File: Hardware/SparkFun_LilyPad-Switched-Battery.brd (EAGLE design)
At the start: 29.8 x 29.7 mm, 13 parts

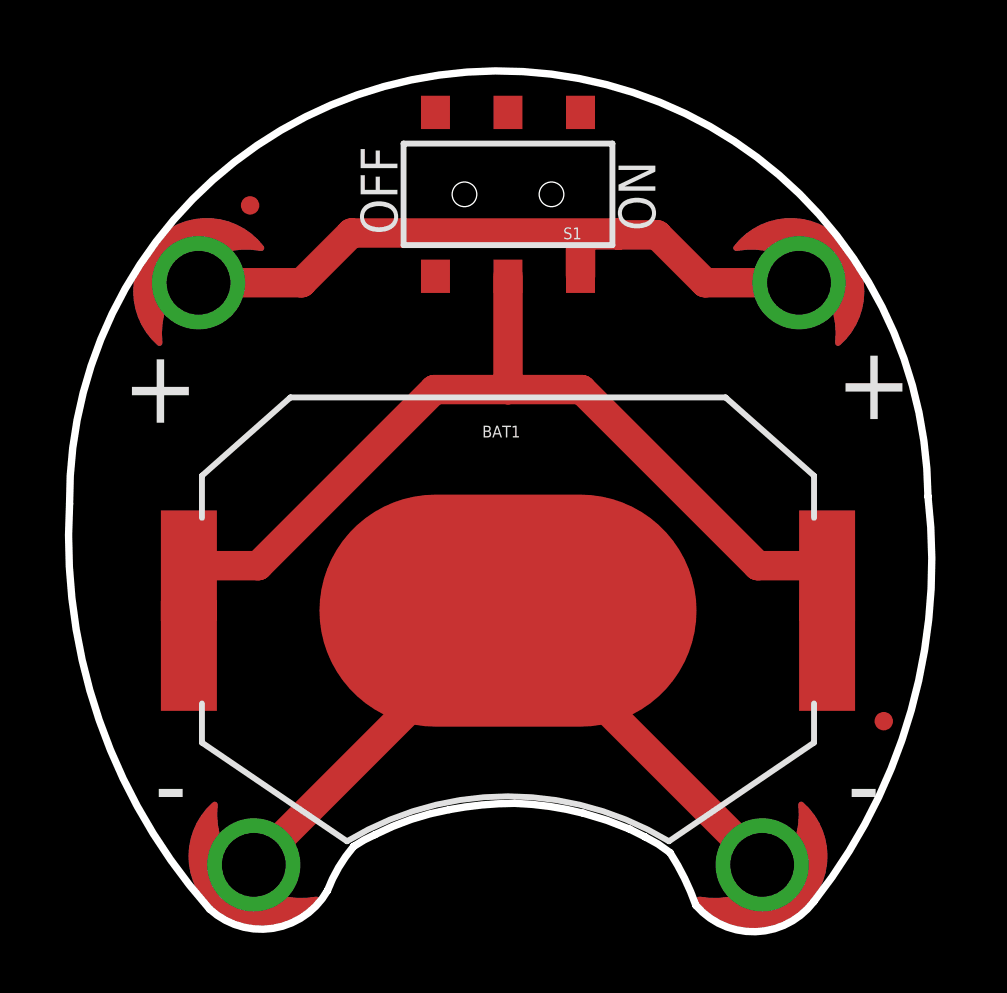
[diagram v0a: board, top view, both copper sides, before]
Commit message: updated board and schematic files
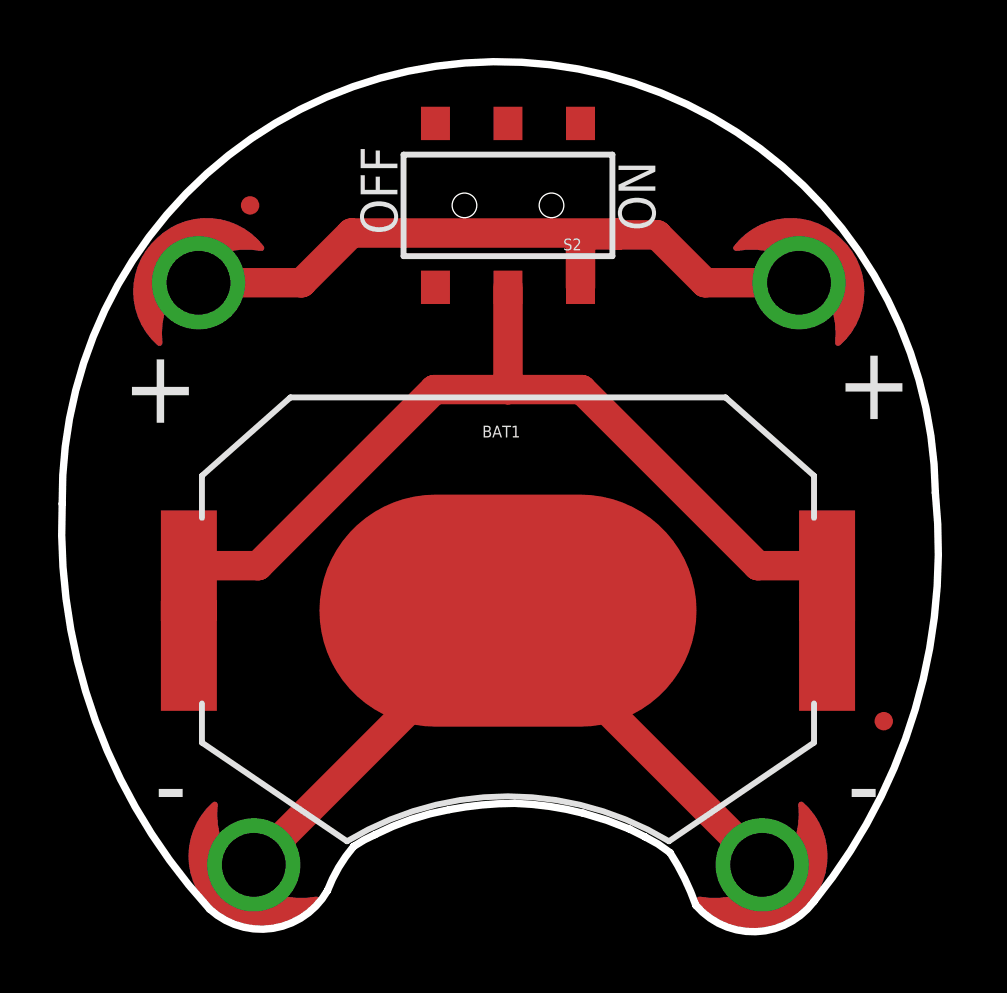
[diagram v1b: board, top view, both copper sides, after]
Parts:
- removed S1: Switch, SparkFun:AYZ0202
- added S2: (no value), SparkFun-Electromechanical:AYZ0202
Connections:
- net N$1: now also S2.1; no longer S1.1
- net N$3: now also S2.2; no longer S1.2
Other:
- board size 29.8 x 29.7 mm -> 30.2 x 30 mm
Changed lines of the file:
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@@
 <setting verticaltext="up"/>
 </settings>
-<grid distance="0.0125" unitdist="inch" unit="inch" style="lines" multiple="1" display="yes" altdistance="0.005" altunitdist="inch" altunit="inch"/>
+<grid distance="0.05" unitdist="inch" unit="inch" style="lines" multiple="1" display="yes" altdistance="0.005" altunitdist="inch" altunit="inch"/>
 <layers>
 <layer number="1" name="Top" color="4" fill="1" visible="yes" active="yes"/>
@@
 <text x="19.05" y="26.924" size="1.27" layer="21" font="vector" ratio="15" rot="R270">ON</text>
 <text x="10.16" y="27.432" size="1.27" layer="21" font="vector" ratio="15" rot="R270">OFF</text>
-<wire x1="0.127" y1="15.113" x2="4.953" y2="1.143" width="0.254" layer="20" curve="45"/>
+<wire x1="-0.127" y1="15.113" x2="4.953" y2="1.143" width="0.254" layer="20" curve="45"/>
 <wire x1="4.953" y1="1.143" x2="9.017" y2="1.778" width="0.254" layer="20" curve="103.204965"/>
 <wire x1="9.017" y1="1.778" x2="9.9187" y2="3.302" width="0.254" layer="20" curve="-19.629056"/>
@@
 <wire x1="17.8435" y1="4.445" x2="19.431" y2="3.8989" width="0.254" layer="20" curve="-8.804635"/>
 <wire x1="19.9644" y1="3.6322" x2="20.828" y2="3.0861" width="0.254" layer="20" curve="-13.702835"/>
-<wire x1="29.718" y1="15.367" x2="0.127" y2="15.113" width="0.254" layer="20" curve="180"/>
-<wire x1="29.718" y1="15.367" x2="25.781" y2="1.397" width="0.254" layer="20" curve="-45"/>
+<wire x1="29.972" y1="15.494" x2="-0.127" y2="15.113" width="0.254" layer="20" curve="180"/>
+<wire x1="29.972" y1="15.494" x2="25.781" y2="1.397" width="0.254" layer="20" curve="-45"/>
 <wire x1="25.781" y1="1.397" x2="21.717" y2="1.27" width="0.254" layer="20" curve="-102.203889"/>
 <wire x1="21.717" y1="1.27" x2="20.828" y2="3.0861" width="0.254" layer="20" curve="13.355078"/>
@@
 <element name="ST4" library="LilyPad-Wearables" package="PETAL-SMALL-2SIDE" value="SEWTAP6" x="25.273" y="22.733" rot="R137"/>
 <element name="U$5" library="LilyPad-Wearables" package="LOGO-LILYPAD" value="LOGO-LPLP" x="15.24" y="15.24" rot="MR0"/>
-<element name="S1" library="SparkFun" package="AYZ0202" value="Switch" x="15.24" y="25.781" rot="R180"/>
 <element name="BAT1" library="SparkFun-Electromechanical" package="BATTCON_20MM_4LEGS" value="20mm coincell" x="15.24" y="11.43">
 <attribute name="PROD_ID" value="BATT-10373" x="15.24" y="11.43" size="1.778" layer="27" display="off"/>
@@
 <element name="FRAME1" library="SparkFun-Aesthetics" package="CREATIVE_COMMONS" value="FRAME-LETTER" x="-21.80295625" y="-10.16"/>
 <element name="U$1" library="SparkFun-Aesthetics" package="REVISION" value="REVISION" x="-10.16" y="-12.7"/>
+<element name="S2" library="SparkFun-Electromechanical" package="AYZ0202" value="" x="15.24" y="25.4" rot="R180">
+<attribute name="SF_ID" value="COM-00597" x="15.24" y="25.4" size="1.778" layer="27" font="vector" ratio="15" rot="R180" display="off"/>
+<attribute name="PROD_ID" value="SWCH-08179" x="15.24" y="25.4" size="1.778" layer="27" font="vector" ratio="15" rot="R180" display="off"/>
+</element>
 </elements>
 <signals>
@@
 <contactref element="ST3" pad="1"/>
 <contactref element="ST4" pad="1"/>
-<contactref element="S1" pad="1"/>
-<wire x1="17.74" y1="22.956" x2="17.74" y2="24.344" width="1.016" layer="1"/>
-<wire x1="17.74" y1="24.344" x2="17.78" y2="24.384" width="1.016" layer="1"/>
 <wire x1="17.78" y1="24.384" x2="19.05" y2="24.384" width="1.016" layer="1"/>
 <wire x1="19.05" y1="24.384" x2="20.3835" y2="24.384" width="1.016" layer="1"/>
@@
 <wire x1="8.128" y1="22.733" x2="9.8425" y2="24.4475" width="1.016" layer="1"/>
 <wire x1="22.0345" y1="22.733" x2="20.3835" y2="24.384" width="1.016" layer="1"/>
+<contactref element="S2" pad="1"/>
+<wire x1="17.74" y1="22.575" x2="17.74" y2="24.344" width="1.016" layer="1"/>
+<wire x1="17.74" y1="24.344" x2="17.78" y2="24.384" width="1.016" layer="1"/>
 </signal>
 <signal name="N$3">
-<contactref element="S1" pad="2"/>
 <contactref element="BAT1" pad="POSITIVE@1"/>
 <contactref element="BAT1" pad="POSITIVE@2"/>
@@
 <wire x1="6.63" y1="12.98" x2="12.7" y2="19.05" width="1.016" layer="1"/>
 <wire x1="12.7" y1="19.05" x2="15.24" y2="19.05" width="1.016" layer="1"/>
+<contactref element="S2" pad="2"/>
 <wire x1="15.24" y1="19.05" x2="17.78" y2="19.05" width="1.016" layer="1"/>
-<wire x1="15.24" y1="22.956" x2="15.24" y2="19.05" width="1.016" layer="1"/>
+<wire x1="15.24" y1="22.575" x2="15.24" y2="19.05" width="1.016" layer="1"/>
 </signal>
 </signals>
+<errors>
+</errors>
 </board>
 </drawing>
